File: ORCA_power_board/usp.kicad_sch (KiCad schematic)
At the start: 52 parts, among them J21 Conn_01x02, Q5 TJ60S04M3L, U10 HY2112, U11 AP64502, U12 TPS61230A__board, U3 CN3058E, U9 FS8205A

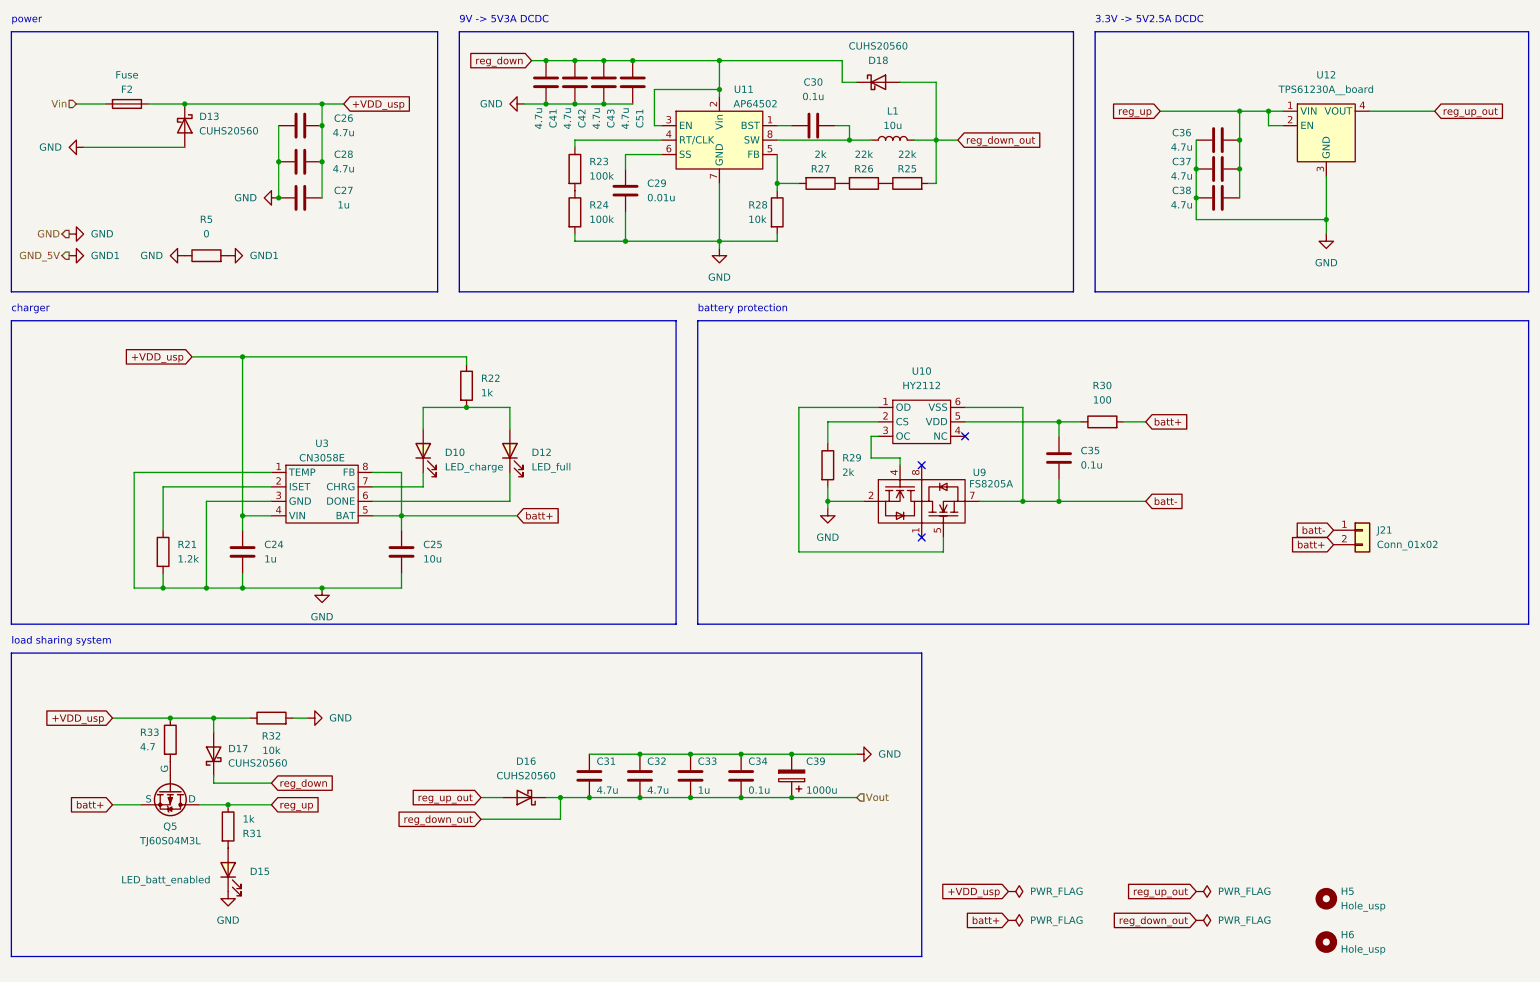
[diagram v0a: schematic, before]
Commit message: complete power_board
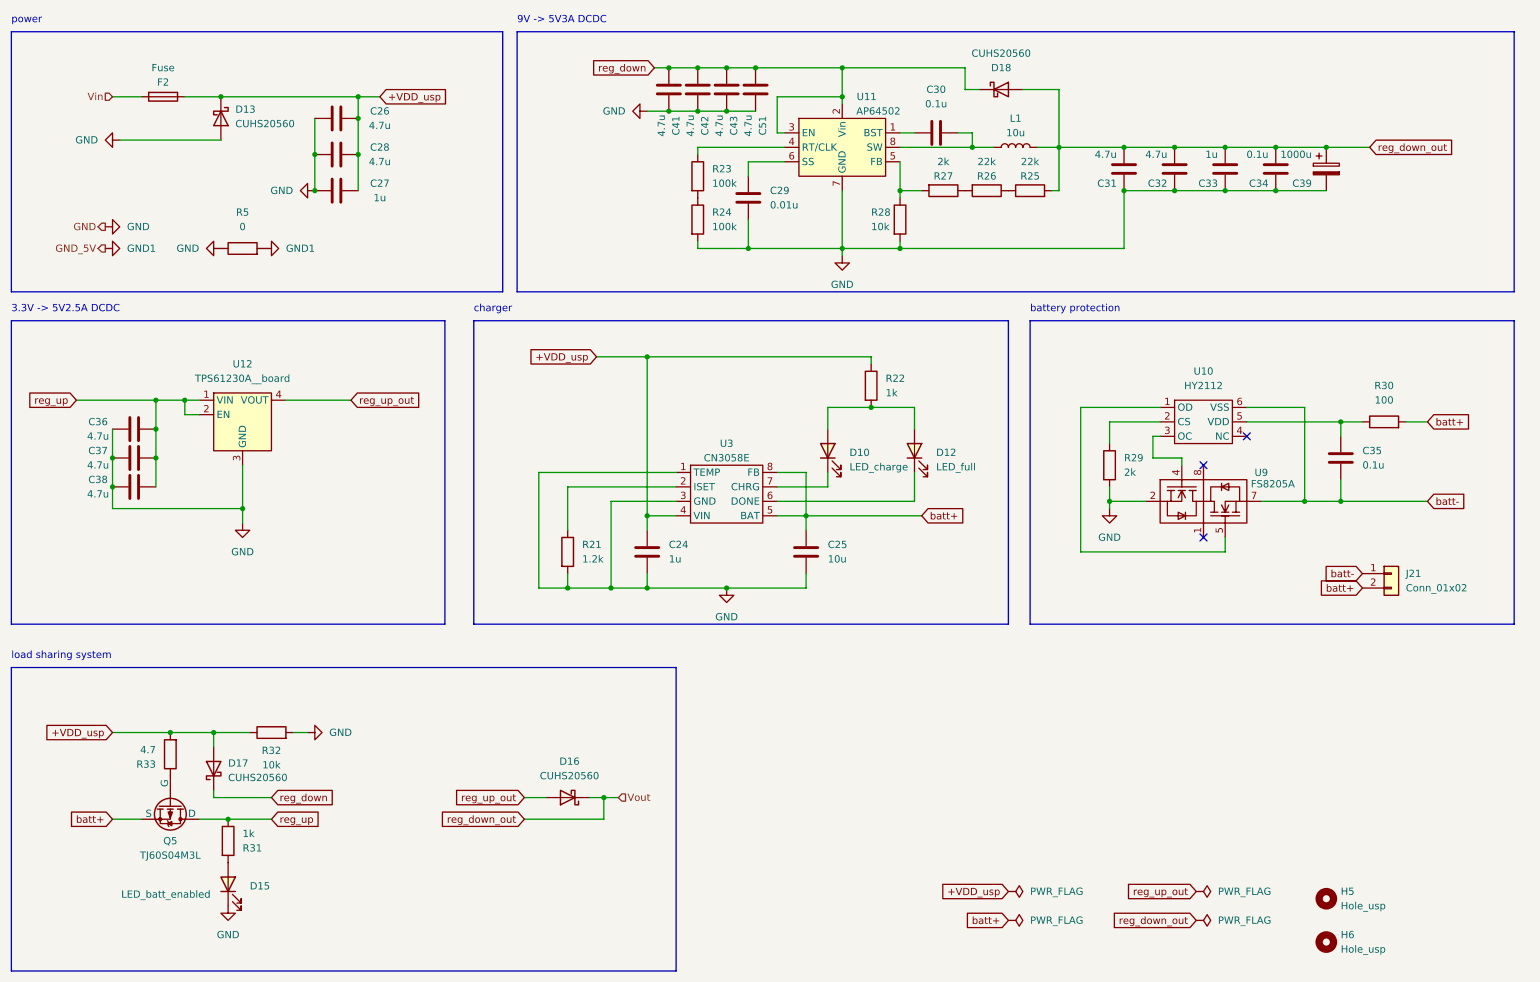
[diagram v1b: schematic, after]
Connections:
- net +VDD_usp: now also R33.2; no longer R33.1
- net at Q5.2 (G): now also R33.1; no longer R33.2
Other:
- moved on the sheet: C24, C25, C26, C27, C28, C29, C30, C31, C32, C33, C34, C35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
